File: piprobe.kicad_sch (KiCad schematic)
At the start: 30 parts, among them J1 USB_C_Receptacle_USB2.0, J2 Conn_01x03_Male, J3 Conn_01x06_Male, J4 Conn_01x10_Male, J5 Conn_01x10_Male, J6 Conn_01x06_Male, U1 TPS63020, U2 RP2040, U3 W25Q32JVZP, Y1 Crystal_GND24_Small

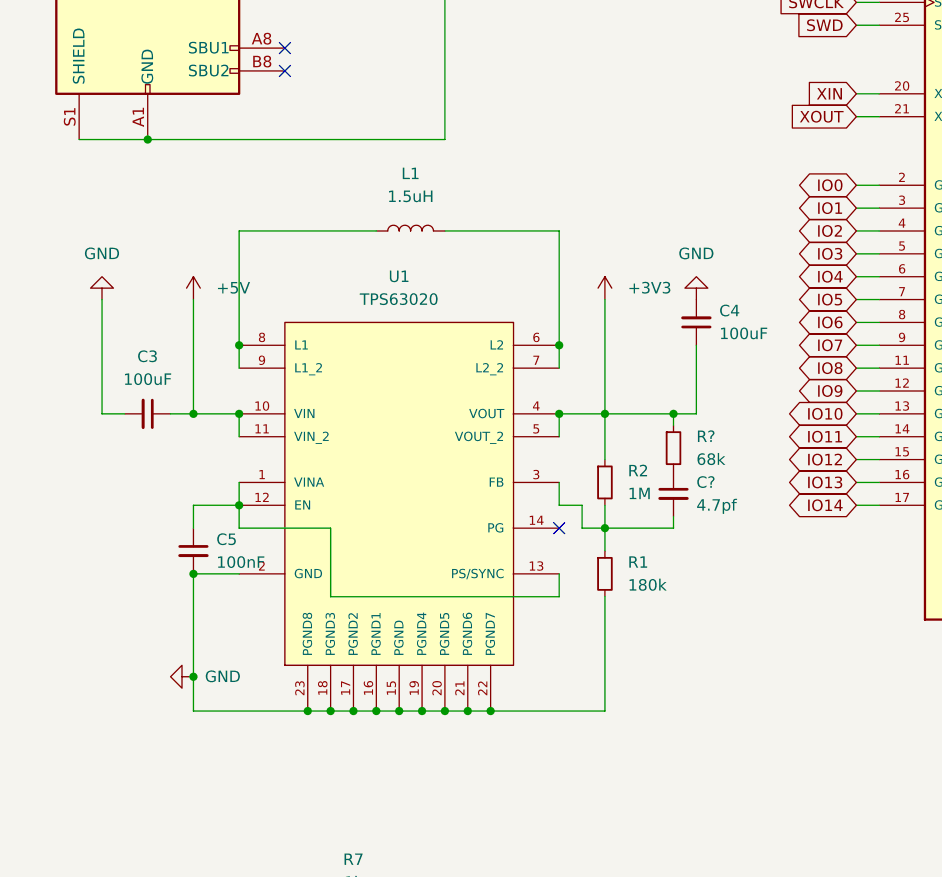
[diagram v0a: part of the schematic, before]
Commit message: ldo
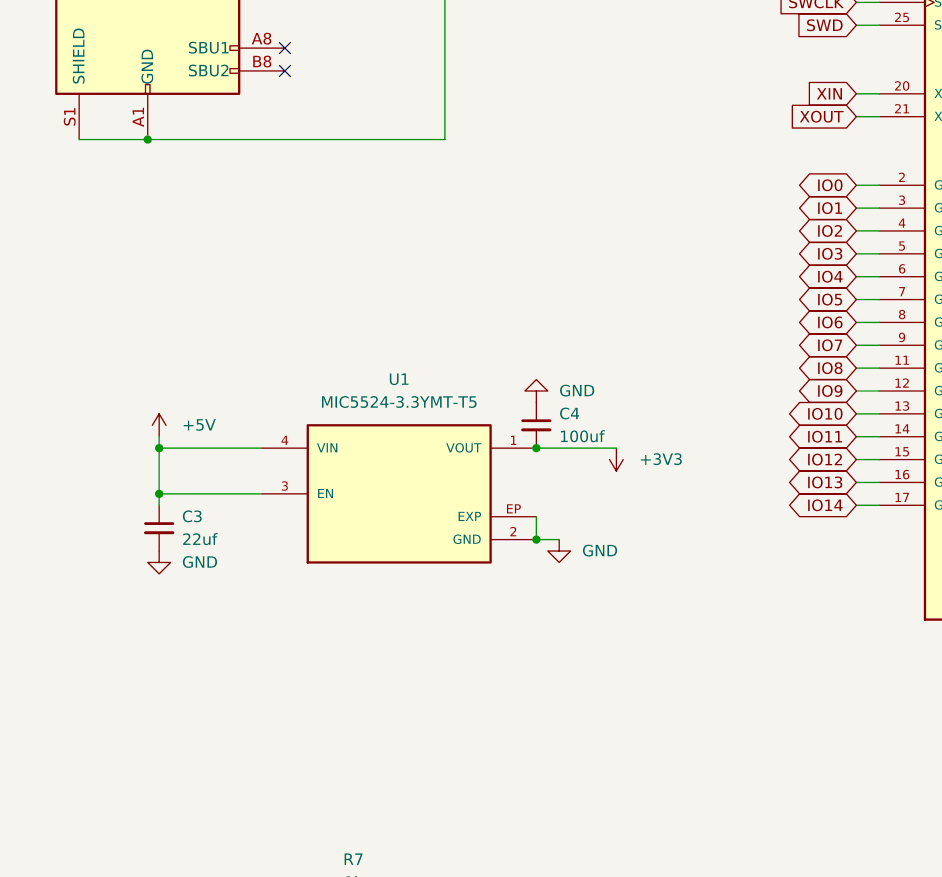
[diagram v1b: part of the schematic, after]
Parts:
- removed C5: 100nF, Capacitor_SMD:C_0402_1005Metric_Pad0.74x0.62mm_HandSolder, symbol Device:C_Small
- removed C?: 4.7pf, symbol Device:C_Small
- removed L1: 1.5uH, Inductor_SMD:L_0805_2012Metric, symbol Device:L
- removed R1: 180k, Resistor_SMD:R_0402_1005Metric_Pad0.72x0.64mm_HandSolder, symbol Device:R_Small
- removed R2: 1M, Resistor_SMD:R_0402_1005Metric_Pad0.72x0.64mm_HandSolder, symbol Device:R_Small
- removed R?: 68k, symbol Device:R_Small
- removed U1: TPS63020, lib:QFN14-3X4MM, symbol lib:TPS63020
- added U1: MIC5524-3.3YMT-T5, lib:VREG_MIC5524-3.3YMT-T5, symbol lib:MIC5524-3.3YMT-T5
- C3: value 100uF -> 22uf; footprint Capacitor_SMD:C_1206_3216Metric -> Capacitor_SMD:C_0603_1608Metric
- C4: value 100uF -> 100uf
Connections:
- net +3V3: now also C4.2, U1.1 (VOUT); no longer C4.1
- net +5V: now also U1.3 (EN), U1.4 (VIN)
- net GND: now also C4.1, U1.2 (GND), U1.EP (EXP); no longer C4.2
- no-connect marks 5 -> 4
